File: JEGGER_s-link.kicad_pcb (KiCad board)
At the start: 2 copper layers, 44.8 x 16.3 mm, 38 parts, among them J1 USB, J2 Tag-Connect, J3 STM_DEBUG, J4 OUT, J5 STLINK_UART, U1 USBLC6-2P6, U2 AP2112K-3.3, U3 STM32F103CBTx, Y1 8Mhz

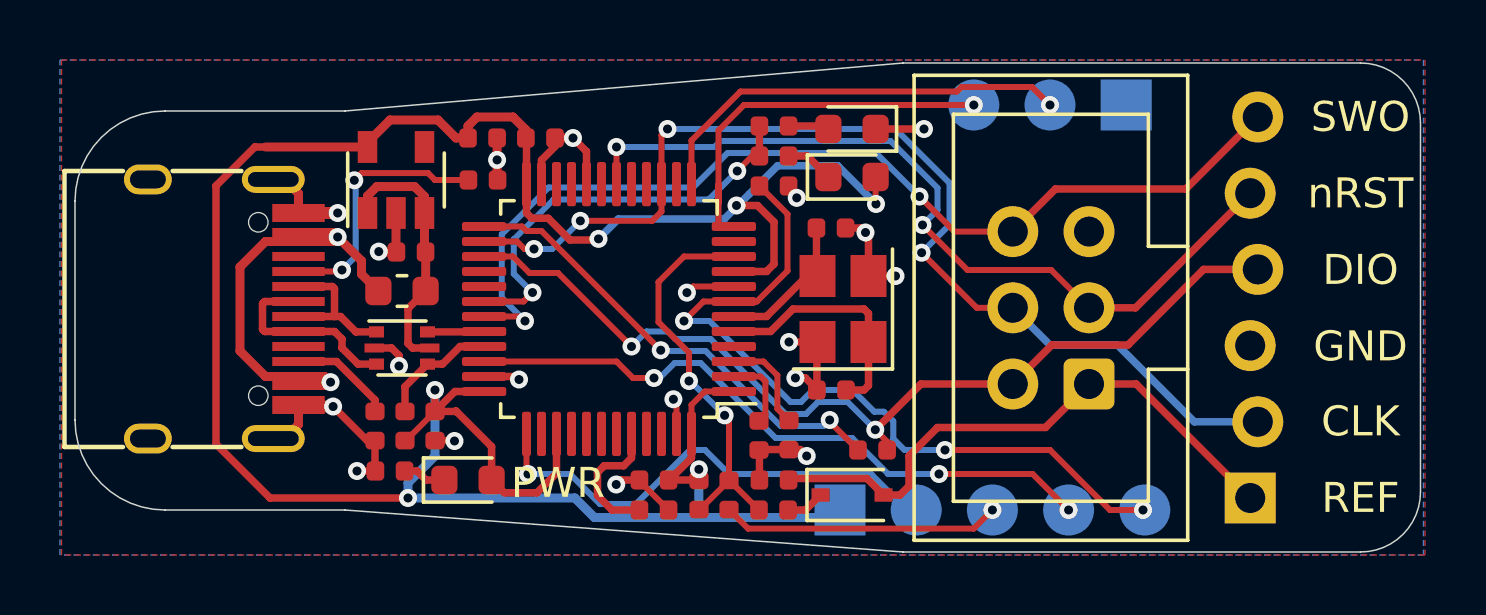
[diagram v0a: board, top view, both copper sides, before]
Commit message: generated gerbers
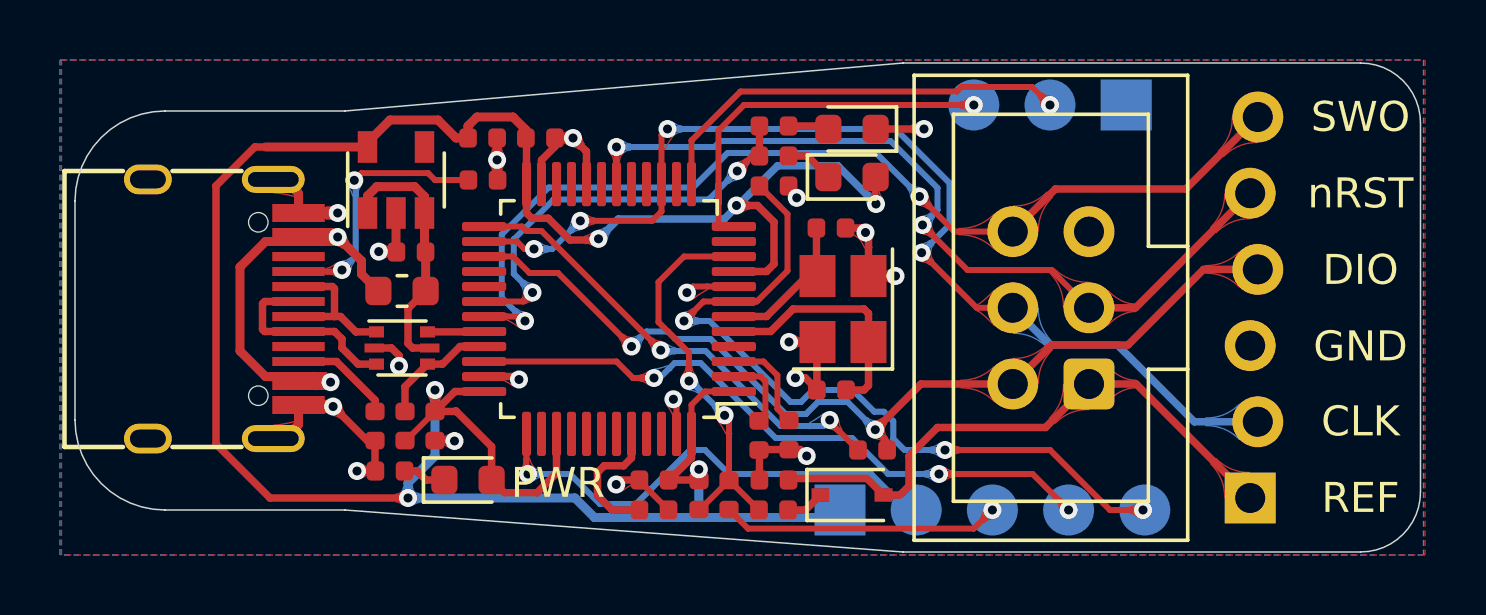
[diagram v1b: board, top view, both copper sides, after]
